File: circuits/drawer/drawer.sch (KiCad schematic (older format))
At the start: 7 parts

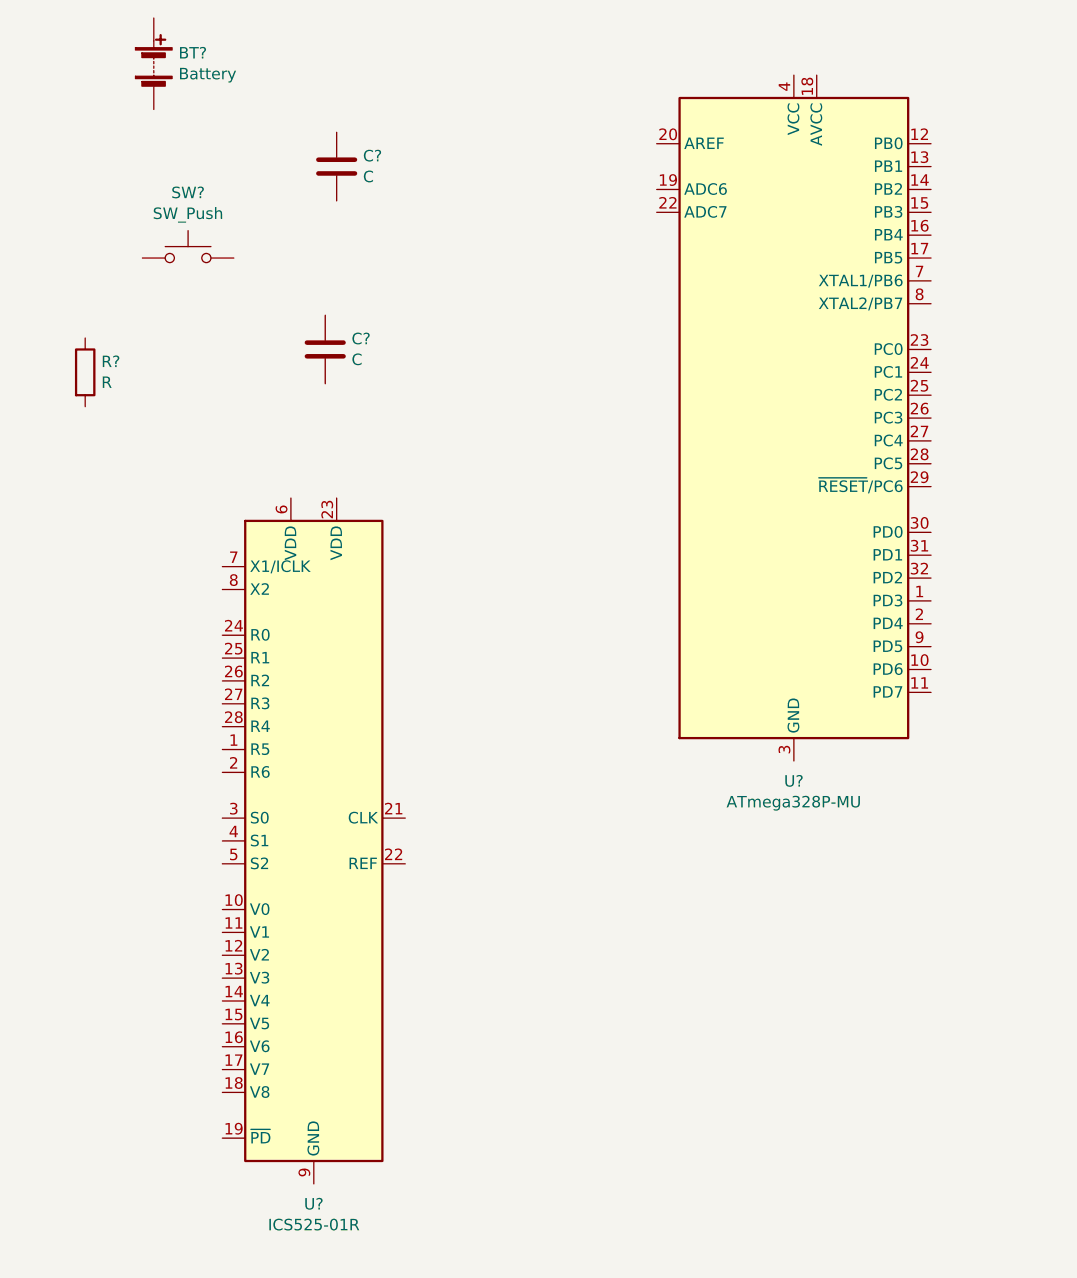
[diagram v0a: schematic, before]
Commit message: [PATCH] Added components
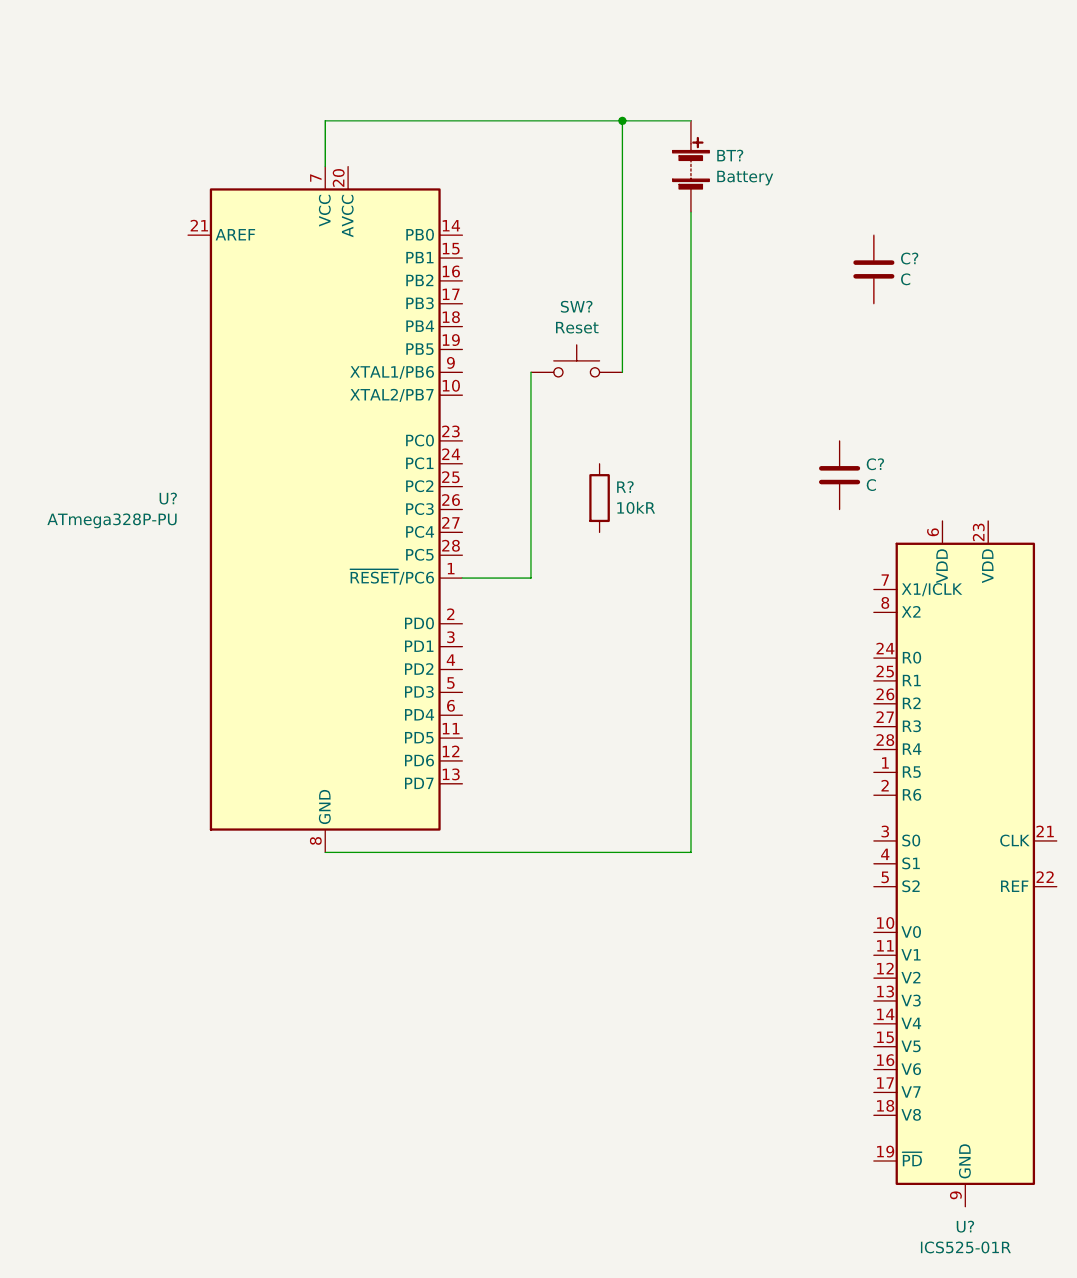
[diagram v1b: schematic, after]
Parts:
- removed U?: ATmega328P-MU, Package_DFN_QFN:QFN-32-1EP_5x5mm_P0.5mm_EP3.1x3.1mm, symbol MCU_Microchip_ATmega:ATmega328P-MU
- added U?: ATmega328P-PU, Package_DIP:DIP-28_W7.62mm, symbol MCU_Microchip_ATmega:ATmega328P-PU
- R?: value R -> 10kR
- SW?: value SW_Push -> Reset
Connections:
- net at BT?.1 (+): now also SW?.2, U?.7 (VCC)
- net at BT?.2 (-): now also U?.22 (GND), U?.8 (GND)
- net at SW?.1: now also U?.1 (~RESET~/PC6)
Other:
- moved on the sheet: BT?, C?, R?, SW?, U?
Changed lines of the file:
@@
 $EndDescr
-$Comp
-L MCU_Microchip_ATmega:ATmega328P-MU U?
-U 1 1 63723DF1
-P 7900 3500
-F 0 "U?" H 7900 1911 50  0000 C CNN
-F 1 "ATmega328P-MU" H 7900 1820 50  0000 C CNN
-F 2 "Package_DFN_QFN:QFN-32-1EP_5x5mm_P0.5mm_EP3.1x3.1mm" H 7900 3500 50  0001 C CIN
-F 3 "http://ww1.microchip.com/downloads/en/DeviceDoc/ATmega328_P%20AVR%20MCU%20with%20picoPower%20Technology%20Data%20Sheet%2040001984A.pdf" H 7900 3500 50  0001 C CNN
-	1    7900 3500
-	1    0    0    -1
-$EndComp
 $Comp
 L Device:C C?
 U 1 1 637262DA
-P 5900 2400
-F 0 "C?" H 6015 2446 50  0000 L CNN
-F 1 "C" H 6015 2355 50  0000 L CNN
-F 2 "" H 5938 2250 50  0001 C CNN
-F 3 "~" H 5900 2400 50  0001 C CNN
-	1    5900 2400
+P 8250 2850
+F 0 "C?" H 8365 2896 50  0000 L CNN
+F 1 "C" H 8365 2805 50  0000 L CNN
+F 2 "" H 8288 2700 50  0001 C CNN
+F 3 "~" H 8250 2850 50  0001 C CNN
+	1    8250 2850
 	1    0    0    -1
 $EndComp
@@
 L Device:C C?
 U 1 1 63726A33
-P 5850 3200
-F 0 "C?" H 5965 3246 50  0000 L CNN
-F 1 "C" H 5965 3155 50  0000 L CNN
-F 2 "" H 5888 3050 50  0001 C CNN
-F 3 "~" H 5850 3200 50  0001 C CNN
-	1    5850 3200
+P 8100 3750
+F 0 "C?" H 8215 3796 50  0000 L CNN
+F 1 "C" H 8215 3705 50  0000 L CNN
+F 2 "" H 8138 3600 50  0001 C CNN
+F 3 "~" H 8100 3750 50  0001 C CNN
+	1    8100 3750
 	1    0    0    -1
 $EndComp
@@
 L Device:Battery BT?
 U 1 1 63726FB9
-P 5100 1950
-F 0 "BT?" H 5208 1996 50  0000 L CNN
-F 1 "Battery" H 5208 1905 50  0000 L CNN
-F 2 "" V 5100 2010 50  0001 C CNN
-F 3 "~" V 5100 2010 50  0001 C CNN
-	1    5100 1950
+P 7450 2400
+F 0 "BT?" H 7558 2446 50  0000 L CNN
+F 1 "Battery" H 7558 2355 50  0000 L CNN
+F 2 "" V 7450 2460 50  0001 C CNN
+F 3 "~" V 7450 2460 50  0001 C CNN
+	1    7450 2400
 	1    0    0    -1
 $EndComp
@@
 L Device:R R?
 U 1 1 63727A35
-P 4800 3300
-F 0 "R?" H 4870 3346 50  0000 L CNN
-F 1 "R" H 4870 3255 50  0000 L CNN
-F 2 "" V 4730 3300 50  0001 C CNN
-F 3 "~" H 4800 3300 50  0001 C CNN
-	1    4800 3300
+P 7050 3850
+F 0 "R?" H 7120 3896 50  0000 L CNN
+F 1 "10kR" H 7120 3805 50  0000 L CNN
+F 2 "" V 6980 3850 50  0001 C CNN
+F 3 "~" H 7050 3850 50  0001 C CNN
+	1    7050 3850
 	1    0    0    -1
 $EndComp
@@
 L Timer_PLL:ICS525-01R U?
 U 1 1 63728339
-P 5800 5350
-F 0 "U?" H 5800 3761 50  0000 C CNN
-F 1 "ICS525-01R" H 5800 3670 50  0000 C CNN
-F 2 "Package_SO:SSOP-28_3.9x9.9mm_P0.635mm" H 5800 3350 50  0001 C CNN
-F 3 "https://www.idt.com/document/dst/525-01-02-datasheet" H 5800 5350 50  0001 C CNN
-	1    5800 5350
+P 8650 5450
+F 0 "U?" H 8650 3861 50  0000 C CNN
+F 1 "ICS525-01R" H 8650 3770 50  0000 C CNN
+F 2 "Package_SO:SSOP-28_3.9x9.9mm_P0.635mm" H 8650 3450 50  0001 C CNN
+F 3 "https://www.idt.com/document/dst/525-01-02-datasheet" H 8650 5450 50  0001 C CNN
+	1    8650 5450
 	1    0    0    -1
 $EndComp
@@
 L Switch:SW_Push SW?
 U 1 1 63729837
-P 5250 2800
-F 0 "SW?" H 5250 3085 50  0000 C CNN
-F 1 "SW_Push" H 5250 2994 50  0000 C CNN
-F 2 "" H 5250 3000 50  0001 C CNN
-F 3 "~" H 5250 3000 50  0001 C CNN
-	1    5250 2800
+P 6950 3300
+F 0 "SW?" H 6950 3585 50  0000 C CNN
+F 1 "Reset" H 6950 3494 50  0000 C CNN
+F 2 "" H 6950 3500 50  0001 C CNN
+F 3 "~" H 6950 3500 50  0001 C CNN
+	1    6950 3300
 	1    0    0    -1
 $EndComp
+$Comp
+L MCU_Microchip_ATmega:ATmega328P-PU U?
+U 1 1 6372A681
+P 5850 3900
+F 0 "U?" H 5206 3946 50  0000 R CNN
+F 1 "ATmega328P-PU" H 5206 3855 50  0000 R CNN
+F 2 "Package_DIP:DIP-28_W7.62mm" H 5850 3900 50  0001 C CIN
+F 3 "http://ww1.microchip.com/downloads/en/DeviceDoc/ATmega328_P%20AVR%20MCU%20with%20picoPower%20Technology%20Data%20Sheet%2040001984A.pdf" H 5850 3900 50  0001 C CNN
+	1    5850 3900
+	1    0    0    -1
+$EndComp
+Wire Wire Line
+	6450 4200 6750 4200
+Wire Wire Line
+	6750 4200 6750 3300
+Wire Wire Line
+	7450 2200 7150 2200
+Wire Wire Line
+	5850 2200 5850 2400
+Wire Wire Line
+	7450 2600 7450 5400
+Wire Wire Line
+	7450 5400 5850 5400
+Wire Wire Line
+	7150 3300 7150 2200
+Connection ~ 7150 2200
+Wire Wire Line
+	7150 2200 5850 2200
 $EndSCHEMATC
